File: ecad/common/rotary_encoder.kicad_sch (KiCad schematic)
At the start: 2 parts, among them SW1 PEL12T

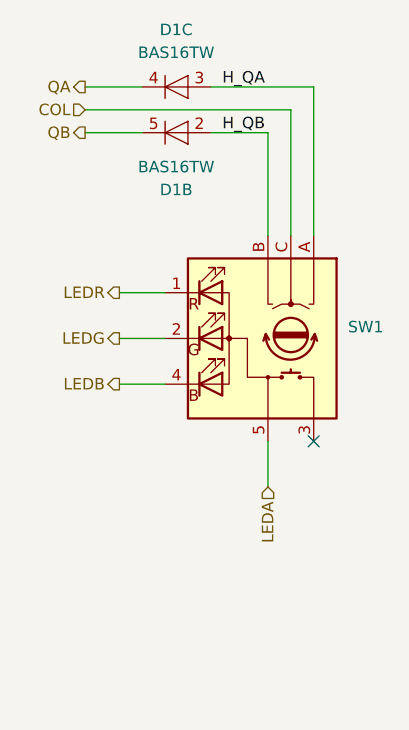
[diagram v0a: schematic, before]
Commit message: [WIP] Layouting a matric led driver
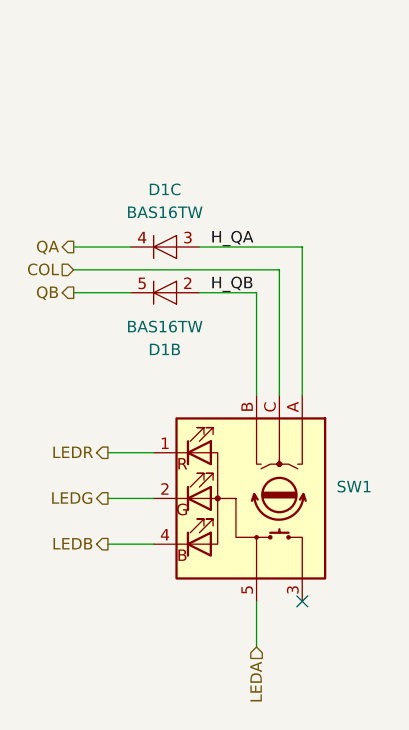
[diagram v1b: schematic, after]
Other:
- moved on the sheet: D1B, D1C, SW1
